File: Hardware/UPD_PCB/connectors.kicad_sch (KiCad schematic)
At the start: 23 parts, among them J1 Screw_Terminal_01x02, J10 Screw_Terminal_01x02, J2 Screw_Terminal_01x02, J3 Screw_Terminal_01x02, J4 Screw_Terminal_01x02, J5 Screw_Terminal_01x02, J6 Screw_Terminal_01x02, J7 Screw_Terminal_01x02, J8 Screw_Terminal_01x02, J9 Screw_Terminal_01x02

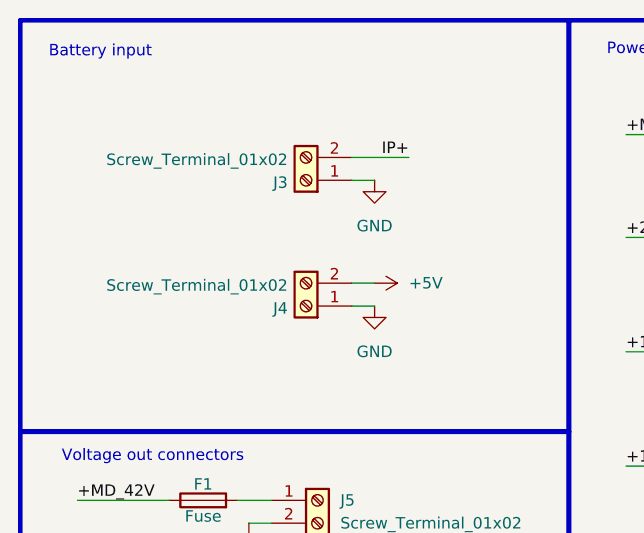
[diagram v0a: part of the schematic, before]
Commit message: Updated design
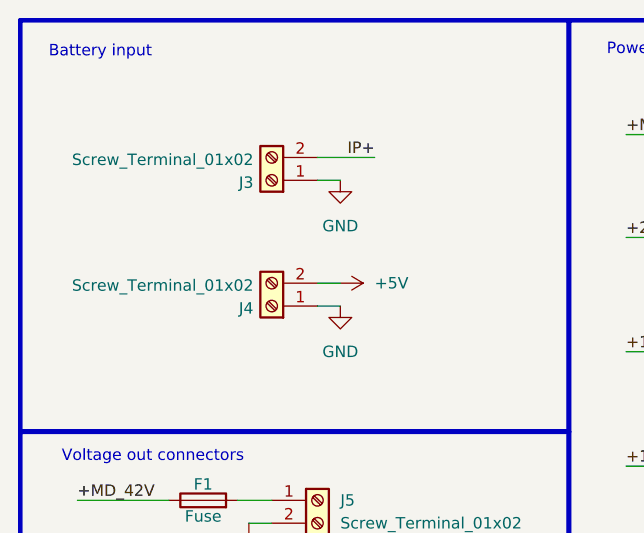
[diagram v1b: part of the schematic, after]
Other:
- moved on the sheet: J3, J4
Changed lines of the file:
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@@
 	(wire
 		(pts
-			(xy 63.5 45.72) (xy 69.85 45.72)
+			(xy 59.69 45.72) (xy 66.04 45.72)
 		)
 		(stroke
@@
 	(wire
 		(pts
-			(xy 63.5 62.23) (xy 66.04 62.23)
+			(xy 59.69 62.23) (xy 62.23 62.23)
 		)
 		(stroke
@@
 	(wire
 		(pts
-			(xy 63.5 59.69) (xy 66.04 59.69)
+			(xy 59.69 59.69) (xy 62.23 59.69)
 		)
 		(stroke
@@
 	(wire
 		(pts
-			(xy 66.04 48.26) (xy 63.5 48.26)
+			(xy 62.23 48.26) (xy 59.69 48.26)
 		)
 		(stroke
@@
 	)
 	(label "IP+"
-		(at 69.85 45.72 180)
+		(at 66.04 45.72 180)
 		(fields_autoplaced yes)
 		(effects
@@
 	(symbol
 		(lib_id "Connector:Screw_Terminal_01x02")
-		(at 58.42 62.23 180)
+		(at 54.61 62.23 180)
 		(unit 1)
 		(exclude_from_sim no)
@@
 		(dnp no)
 		(property "Reference" "J4"
-			(at 56.388 62.484 0)
+			(at 52.578 62.484 0)
 			(effects
 				(font
@@
 		)
 		(property "Value" "Screw_Terminal_01x02"
-			(at 56.388 59.944 0)
+			(at 52.578 59.944 0)
 			(effects
 				(font
@@
 		)
 		(property "Footprint" ""
-			(at 58.42 62.23 0)
+			(at 54.61 62.23 0)
 			(effects
 				(font
@@
 		)
 		(property "Datasheet" "~"
-			(at 58.42 62.23 0)
+			(at 54.61 62.23 0)
 			(effects
 				(font
@@
 		)
 		(property "Description" "Generic screw terminal, single row, 01x02, script generated (kicad-library-utils/schlib/autogen/connector/)"
-			(at 58.42 62.23 0)
+			(at 54.61 62.23 0)
 			(effects
 				(font
@@
 	(symbol
 		(lib_id "power:GND")
-		(at 66.04 62.23 0)
+		(at 62.23 62.23 0)
 		(unit 1)
 		(exclude_from_sim no)
@@
 		(fields_autoplaced yes)
 		(property "Reference" "#PWR058"
-			(at 66.04 68.58 0)
+			(at 62.23 68.58 0)
 			(effects
 				(font
@@
 		)
 		(property "Value" "GND"
-			(at 66.04 67.31 0)
+			(at 62.23 67.31 0)
 			(effects
 				(font
@@
 		)
 		(property "Footprint" ""
-			(at 66.04 62.23 0)
+			(at 62.23 62.23 0)
 			(effects
 				(font
@@
 		)
 		(property "Datasheet" ""
-			(at 66.04 62.23 0)
+			(at 62.23 62.23 0)
 			(effects
 				(font
@@
 		)
 		(property "Description" "Power symbol creates a global label with name \"GND\" , ground"
-			(at 66.04 62.23 0)
+			(at 62.23 62.23 0)
 			(effects
 				(font
@@
 	(symbol
 		(lib_id "power:GND")
-		(at 66.04 48.26 0)
+		(at 62.23 48.26 0)
 		(unit 1)
 		(exclude_from_sim no)
@@
 		(fields_autoplaced yes)
 		(property "Reference" "#PWR056"
-			(at 66.04 54.61 0)
+			(at 62.23 54.61 0)
 			(effects
 				(font
@@
 		)
 		(property "Value" "GND"
-			(at 66.04 53.34 0)
+			(at 62.23 53.34 0)
 			(effects
 				(font
@@
 		)
 		(property "Footprint" ""
-			(at 66.04 48.26 0)
+			(at 62.23 48.26 0)
 			(effects
 				(font
@@
 		)
 		(property "Datasheet" ""
-			(at 66.04 48.26 0)
+			(at 62.23 48.26 0)
 			(effects
 				(font
@@
 		)
 		(property "Description" "Power symbol creates a global label with name \"GND\" , ground"
-			(at 66.04 48.26 0)
+			(at 62.23 48.26 0)
 			(effects
 				(font
@@
 	(symbol
 		(lib_id "Connector:Screw_Terminal_01x02")
-		(at 58.42 48.26 180)
+		(at 54.61 48.26 180)
 		(unit 1)
 		(exclude_from_sim no)
@@
 		(dnp no)
 		(property "Reference" "J3"
-			(at 56.388 48.514 0)
+			(at 52.578 48.514 0)
 			(effects
 				(font
@@
 		)
 		(property "Value" "Screw_Terminal_01x02"
-			(at 56.388 45.974 0)
+			(at 52.578 45.974 0)
 			(effects
 				(font
@@
 		)
 		(property "Footprint" ""
-			(at 58.42 48.26 0)
+			(at 54.61 48.26 0)
 			(effects
 				(font
@@
 		)
 		(property "Datasheet" "~"
-			(at 58.42 48.26 0)
+			(at 54.61 48.26 0)
 			(effects
 				(font
@@
 		)
 		(property "Description" "Generic screw terminal, single row, 01x02, script generated (kicad-library-utils/schlib/autogen/connector/)"
-			(at 58.42 48.26 0)
+			(at 54.61 48.26 0)
 			(effects
 				(font
@@
 	(symbol
 		(lib_id "power:+5V")
-		(at 66.04 59.69 270)
+		(at 62.23 59.69 270)
 		(unit 1)
 		(exclude_from_sim no)
@@
 		(fields_autoplaced yes)
 		(property "Reference" "#PWR057"
+			(at 58.42 59.69 0)
+			(effects
+				(font
+					(size 1.27 1.27)
+				)
+				(hide yes)
+			)
+		)
+		(property "Value" "+5V"
+			(at 66.04 59.6899 90)
+			(effects
+				(font
+					(size 1.27 1.27)
+				)
+				(justify left)
+			)
+		)
+		(property "Footprint" ""
 			(at 62.23 59.69 0)
 			(effects
@@
 			)
 		)
-		(property "Value" "+5V"
-			(at 69.85 59.6899 90)
-			(effects
-				(font
-					(size 1.27 1.27)
-				)
-				(justify left)
-			)
-		)
-		(property "Footprint" ""
-			(at 66.04 59.69 0)
-			(effects
-				(font
-					(size 1.27 1.27)
-				)
-				(hide yes)
-			)
-		)
 		(property "Datasheet" ""
-			(at 66.04 59.69 0)
+			(at 62.23 59.69 0)
 			(effects
 				(font
@@
 		)
 		(property "Description" "Power symbol creates a global label with name \"+5V\""
-			(at 66.04 59.69 0)
-			(effects
-				(font
+			(at 62.23 59.69 0)
+			(effects
+				(font
